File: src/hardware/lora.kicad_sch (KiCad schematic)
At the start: 19 parts

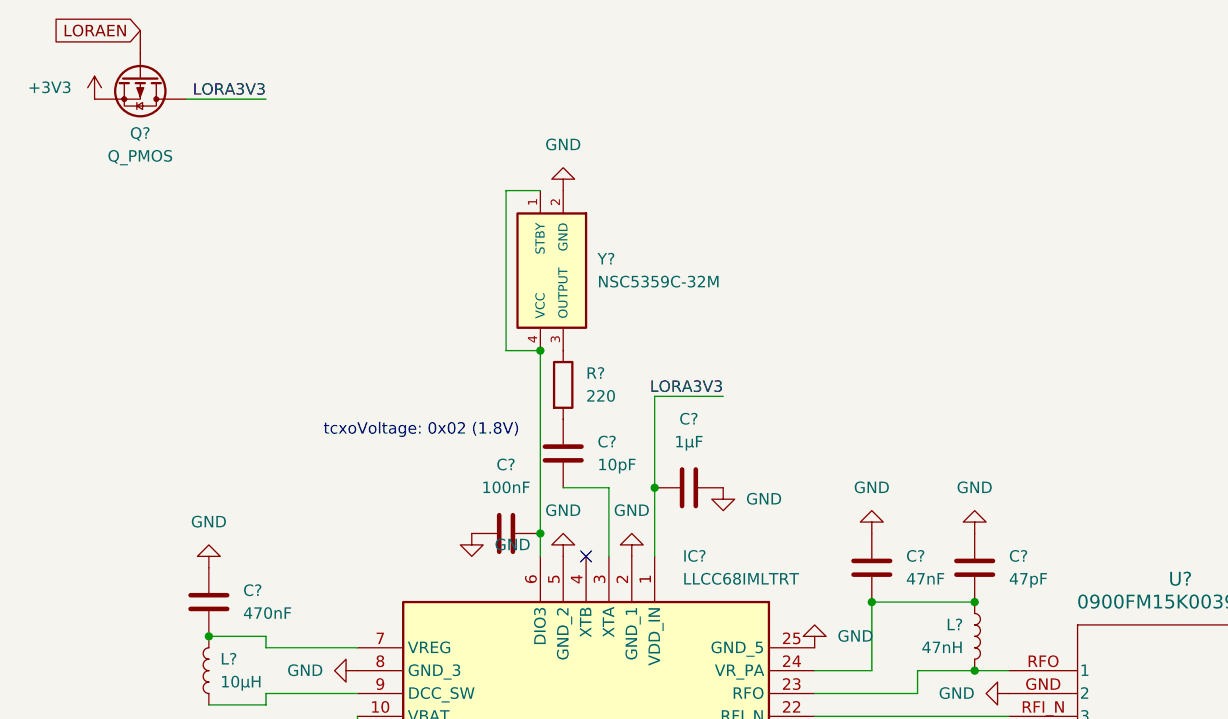
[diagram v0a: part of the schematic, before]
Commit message: LoRa Crystal Optional
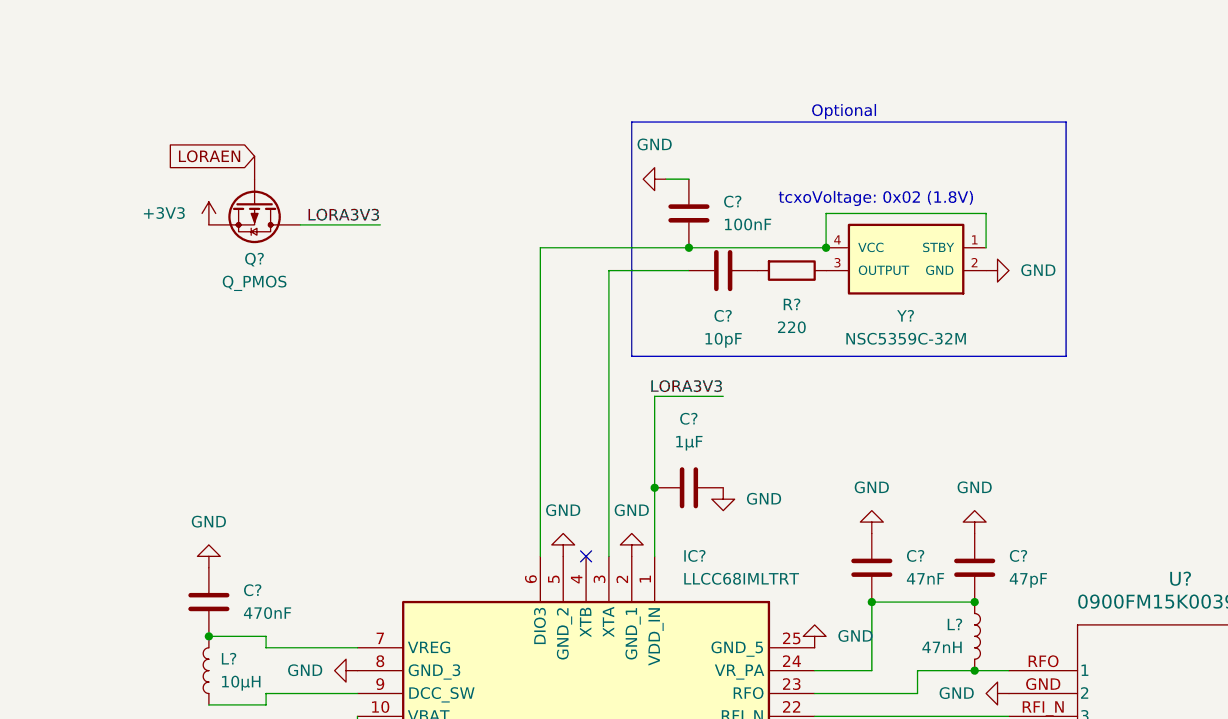
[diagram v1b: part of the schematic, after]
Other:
- note added: "Optional"
- moved on the sheet: C?, Q?, R?, Y?
